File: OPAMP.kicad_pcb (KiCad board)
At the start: 2 copper layers, 33 x 23 mm, 49 parts, among them J1 GH125-S02CCA-00, J2 GH125-S06DCA-00, J3 GH125-S03DCA-00, SW1 DSHP02TSGET, U1 ADG704BRMZ-REEL, U2 AD8421BRZ-RL, U3 OPA2197QDGKRQ1, U4 REF2030AIDDCR

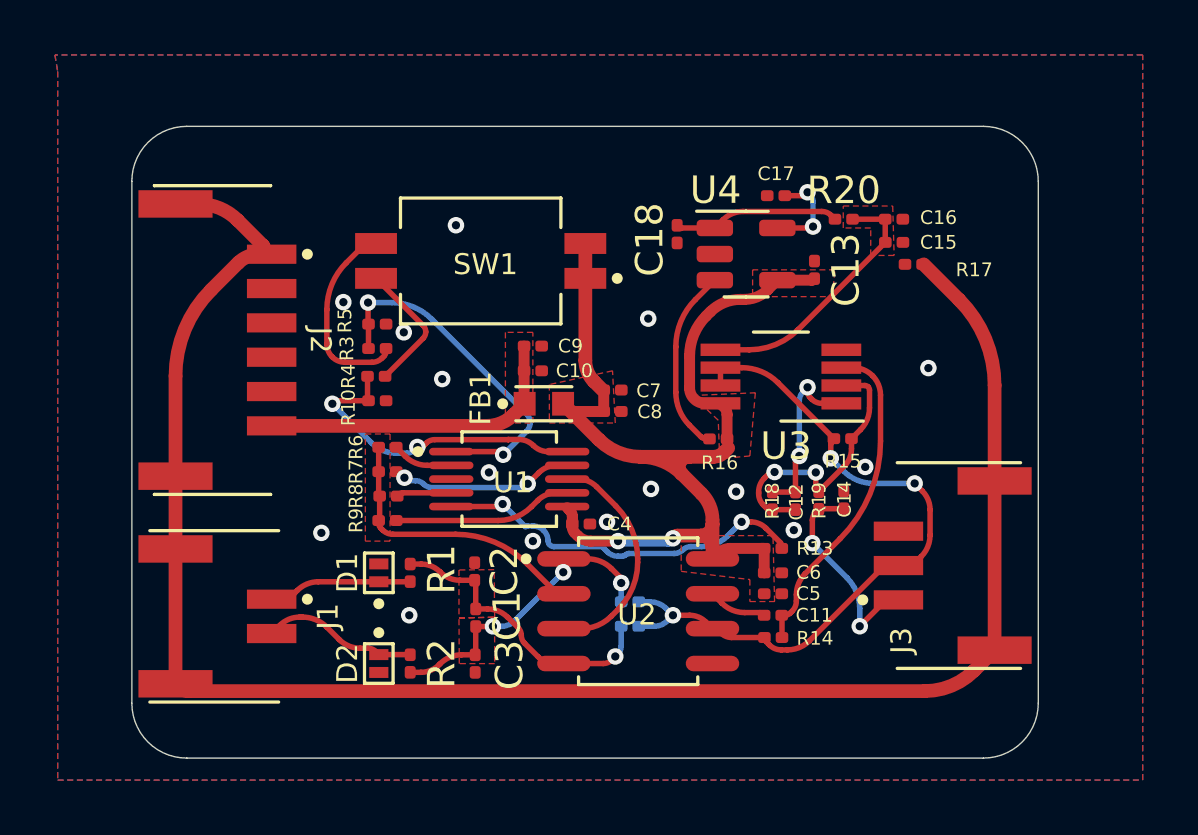
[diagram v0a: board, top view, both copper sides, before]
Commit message: update
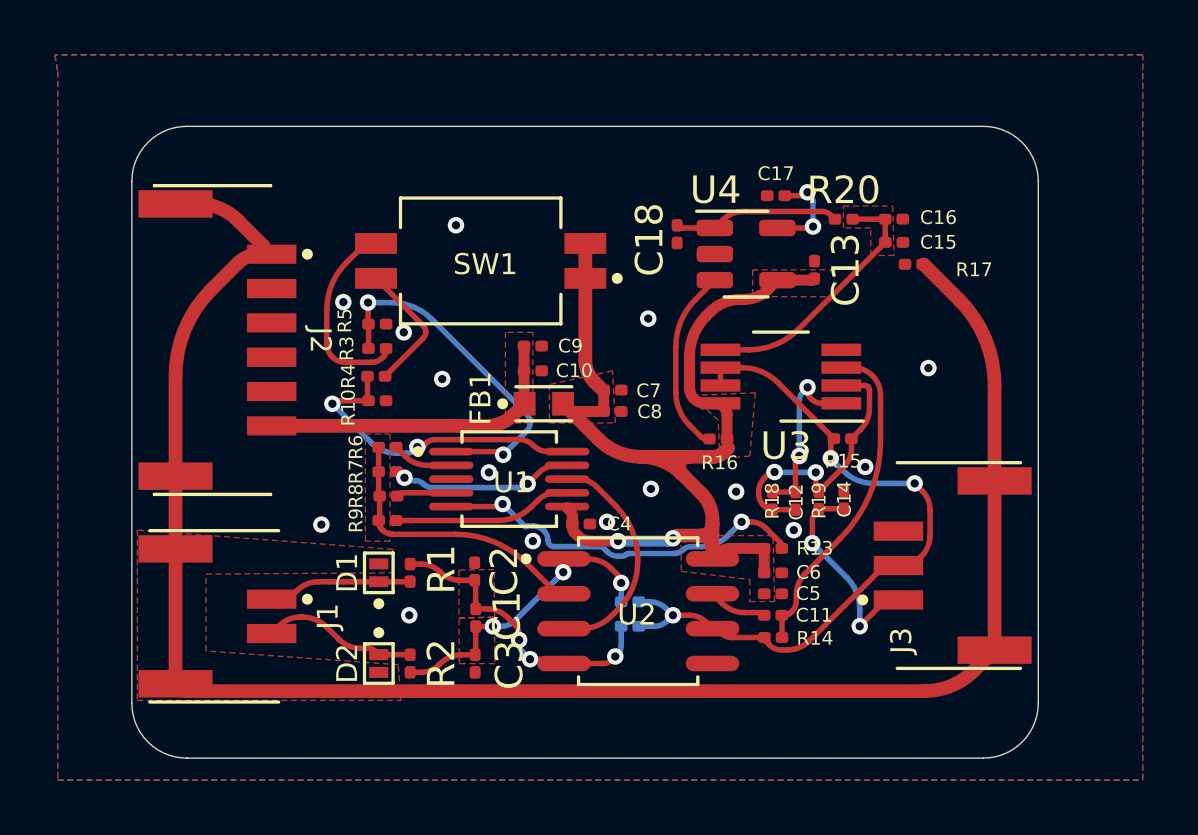
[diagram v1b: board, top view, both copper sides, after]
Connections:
- D1 pad 2: /AGND -> /AGND_SHIELD
- D2 pad 2: /AGND -> /AGND_SHIELD
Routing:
- net /COIL_FILT_P: vias 1 -> 3
- added copper zone on F.Cu, net /AGND_SHIELD
